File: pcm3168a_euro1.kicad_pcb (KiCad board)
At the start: 2 copper layers, 141.8 x 132.5 mm, 271 parts, among them J1 ACJS-MV35-3, J10 Conn_Coaxial, J11 Conn_Coaxial, J12 Conn_Coaxial, J13 Conn_Coaxial, J14 Conn_Coaxial, J15 Conn_Coaxial, J17 ACJS-MV35-3, J18 Conn_02x08_Odd_Even, J19 Conn_Coaxial, J21 ACJS-MV35-3, J22 ACJS-MV35-3, J24 ACJS-MV35-3, J25 ACJS-MV35-3, J26 ACJS-MV35-3, J27 ACJS-MV35-3, J8 Conn_01x02_Pin, J9 Conn_Coaxial, U1 PCM3168APAPR, U11 OPA1637, U12 TLV1117-33, U13 OPA1637, U14 OPA1637, U15 OPA1637, U16 OPA1637, U17 OPA1637, U18 OPA1637, U19 OPA1637, U2 74LVC1G17, U20 OPA1637, U21 OPA1637, U22 OPA1637, U23 OPA1637, U3 74LVC1G17, U4 74LVC1G17, U5 74LVC1G17, U6 74LVC1G17, U8 74LVC1G17, U9 74LVC1G17, Y1 SG-210STF 24.5760ML0

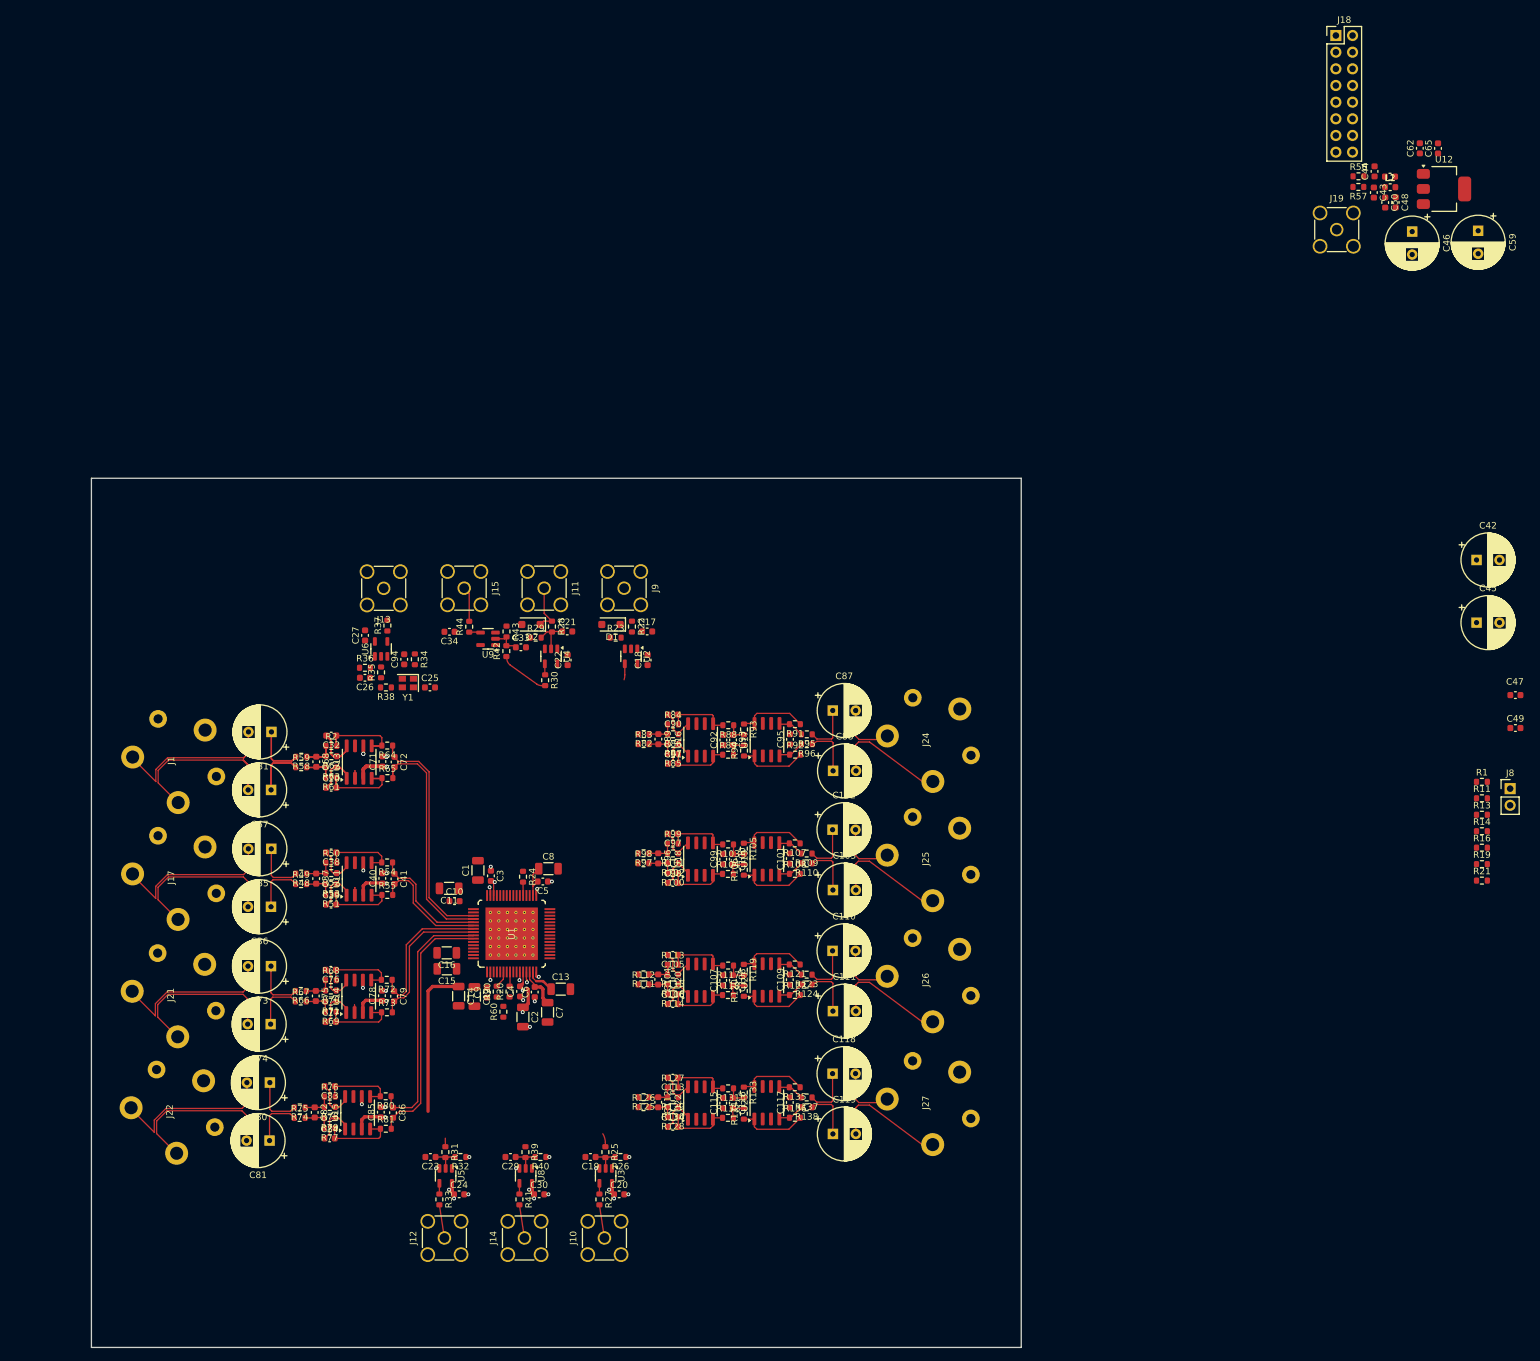
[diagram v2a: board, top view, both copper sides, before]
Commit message: WIP layout
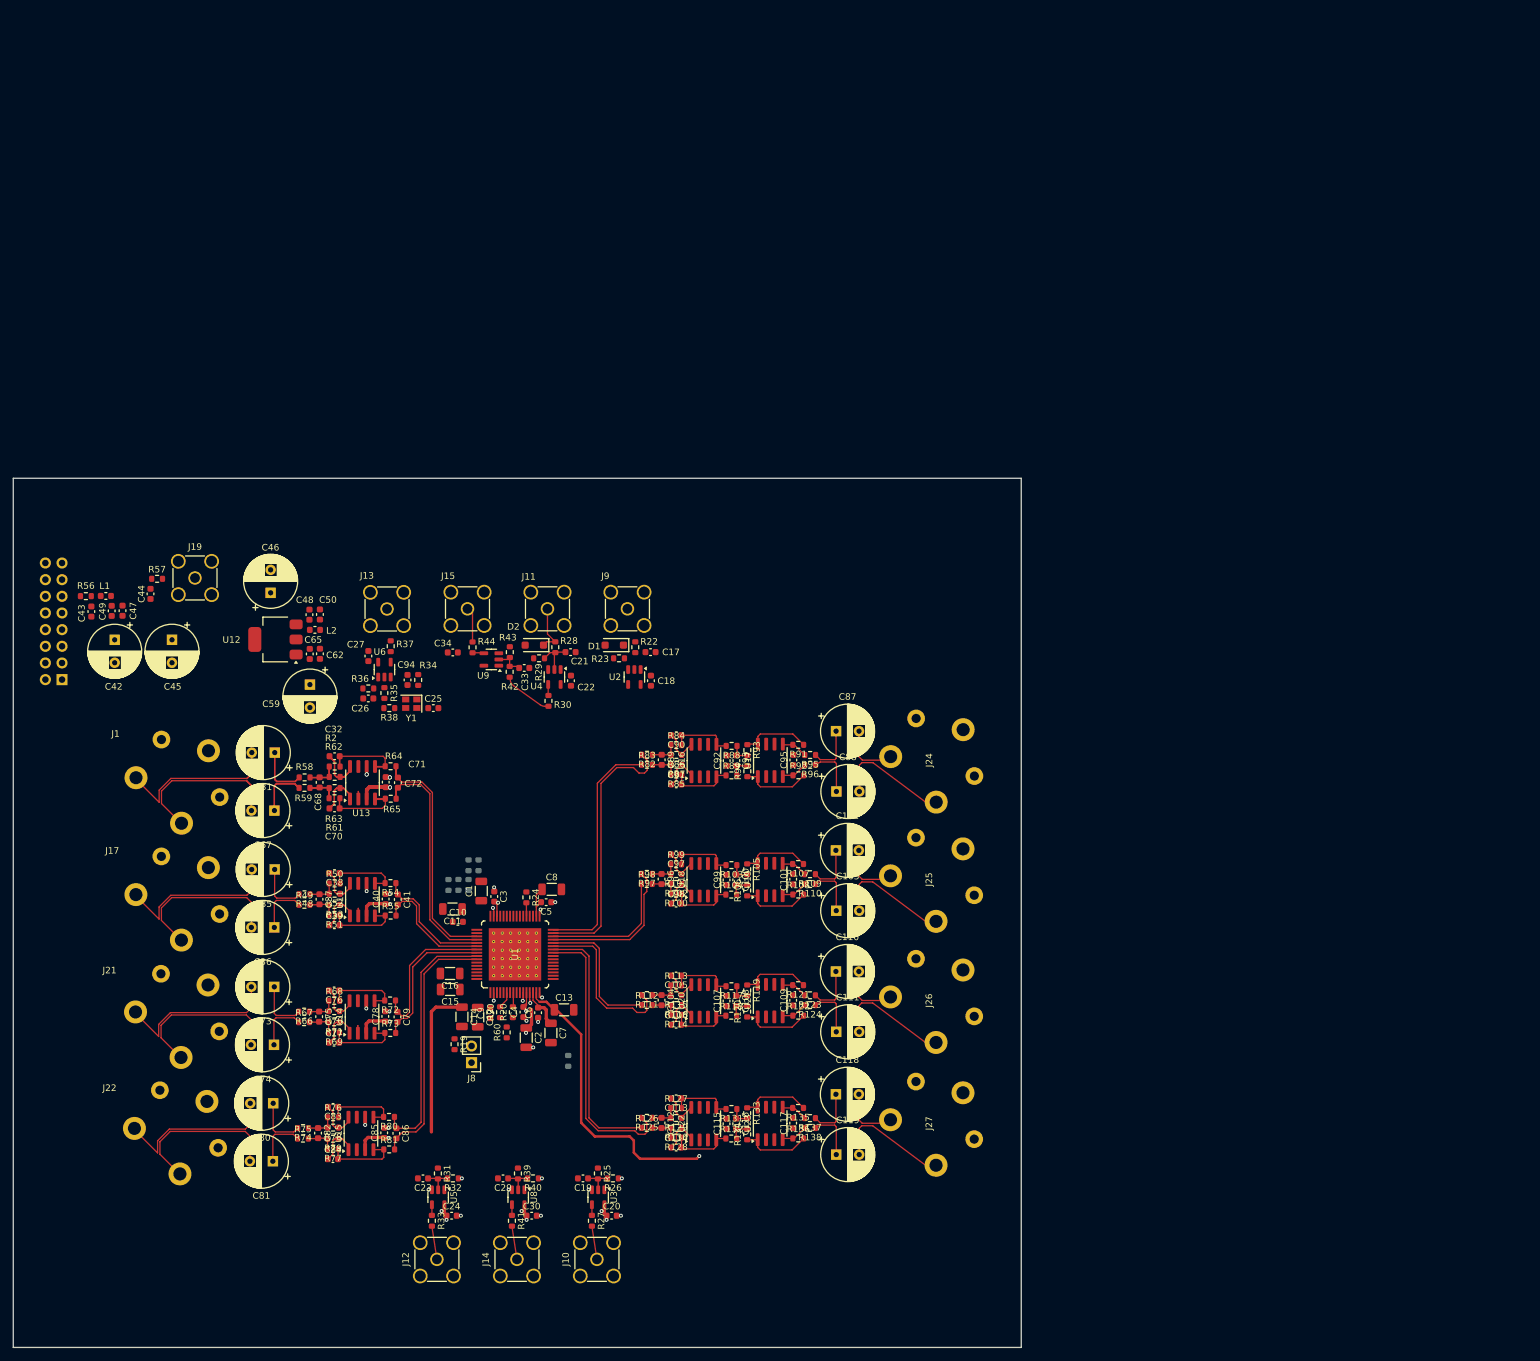
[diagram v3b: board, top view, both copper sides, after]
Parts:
- J18: footprint Connector_PinHeader_2.54mm:PinHeader_2x08_P2.54mm_Vertical -> Connector_PinSocket_2.54mm:PinSocket_2x08_P2.54mm_Vertical; moved to B.Cu
- R1, R11, R13, R14, R16, R21: moved to B.Cu
- moved J18 217.6 mm to (58.2, 115.2)
- moved C49 214.8 mm to (65.7, 104.7), turned to -90 degrees
- moved C47 212.7 mm to (67.4, 104.7), turned to -90 degrees
- moved C42 208.0 mm to (66.2, 109.1), turned to -90 degrees
- moved L1 206.0 mm to (64.8, 102.5)
- moved C43 205.7 mm to (62.6, 104.8)
- moved R56 204.3 mm to (61.8, 102.5)
- moved C45 198.9 mm to (74.9, 109.1), turned to -90 degrees
- moved C44 197.4 mm to (71.7, 102.1), turned to -90 degrees
- moved R57 192.6 mm to (72.7, 99.8), turned to 0 degrees
- moved C59 191.1 mm to (96.0, 116.0)
- moved U12 190.9 mm to (90.7, 109.1), turned to 180 degrees
- moved C65 188.5 mm to (95.9, 111.3), turned to -90 degrees
- moved C62 184.6 mm to (97.5, 111.3), turned to -90 degrees
- moved C46 182.5 mm to (90.0, 102.0), turned to 90 degrees
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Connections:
- C1 pad 1: +3.3V -> VDD
- C2 pad 1: +3.3V -> VDD
- C3 pad 2: +3.3V -> VDD
- C4 pad 2: +3.3V -> VDD
- C59 pad 1: +3.3V -> VDD
- C62 pad 1: +3.3V -> VDD
- C65 pad 1: +3.3V -> VDD
- U1 pad 12: +3.3V -> VDD
- U1 pad 46: +3.3V -> VDD
- U12 pad 2: +3.3V -> VDD
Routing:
- net /VOUT4+: track 0.00 -> 42.8 mm
- net /VOUT1+: track 0.00 -> 40.8 mm
- net Net-(U1-VCOMDA): track 4.39 -> 45.0 mm, vias 0 -> 1
- net /VOUT4-: track 0.00 -> 39.2 mm
- net /VOUT1-: track 0.00 -> 36.5 mm
- net /VOUT3+: track 0.00 -> 25.6 mm
- net /VOUT2+: track 0.00 -> 23.1 mm
- net /VOUT3-: track 0.00 -> 21.7 mm
- net /VOUT2-: track 0.00 -> 20.3 mm
- net +3.3V: track 9.95 -> 0.00 mm, vias 3 -> 0
- net VDD: track 8.64 -> 18.6 mm, vias 6 -> 9
- net Net-(R24-Pad1): track 2.45 -> 0.00 mm
- net /dout1/IN: track 2.04 -> 0.00 mm
- net /lrck_master/IN: track 1.30 -> 0.00 mm
- added copper zone on In2.Cu, net +5V
- added copper zone on In2.Cu, net VDD
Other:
- board size 141.8 x 132.5 mm -> 153.7 x 132.5 mm
- copper layers 2 -> 4

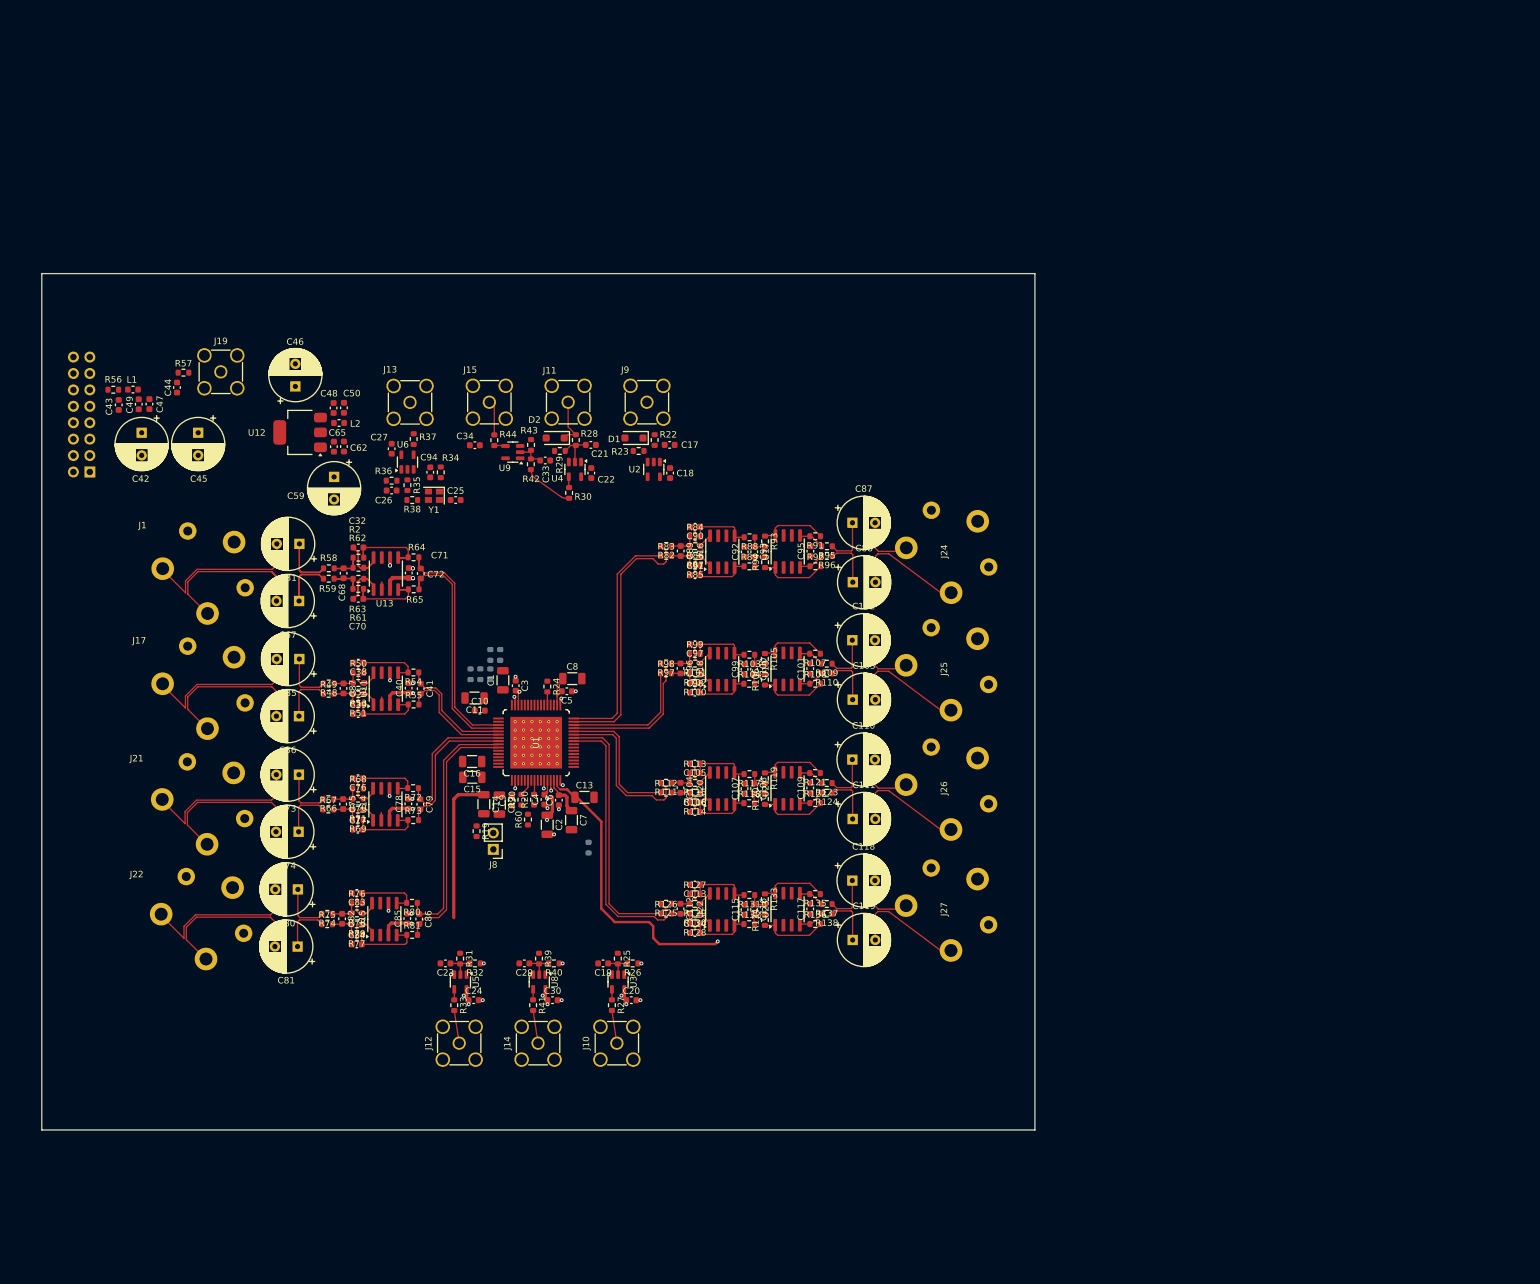
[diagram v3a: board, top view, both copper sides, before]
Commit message: WIP layout
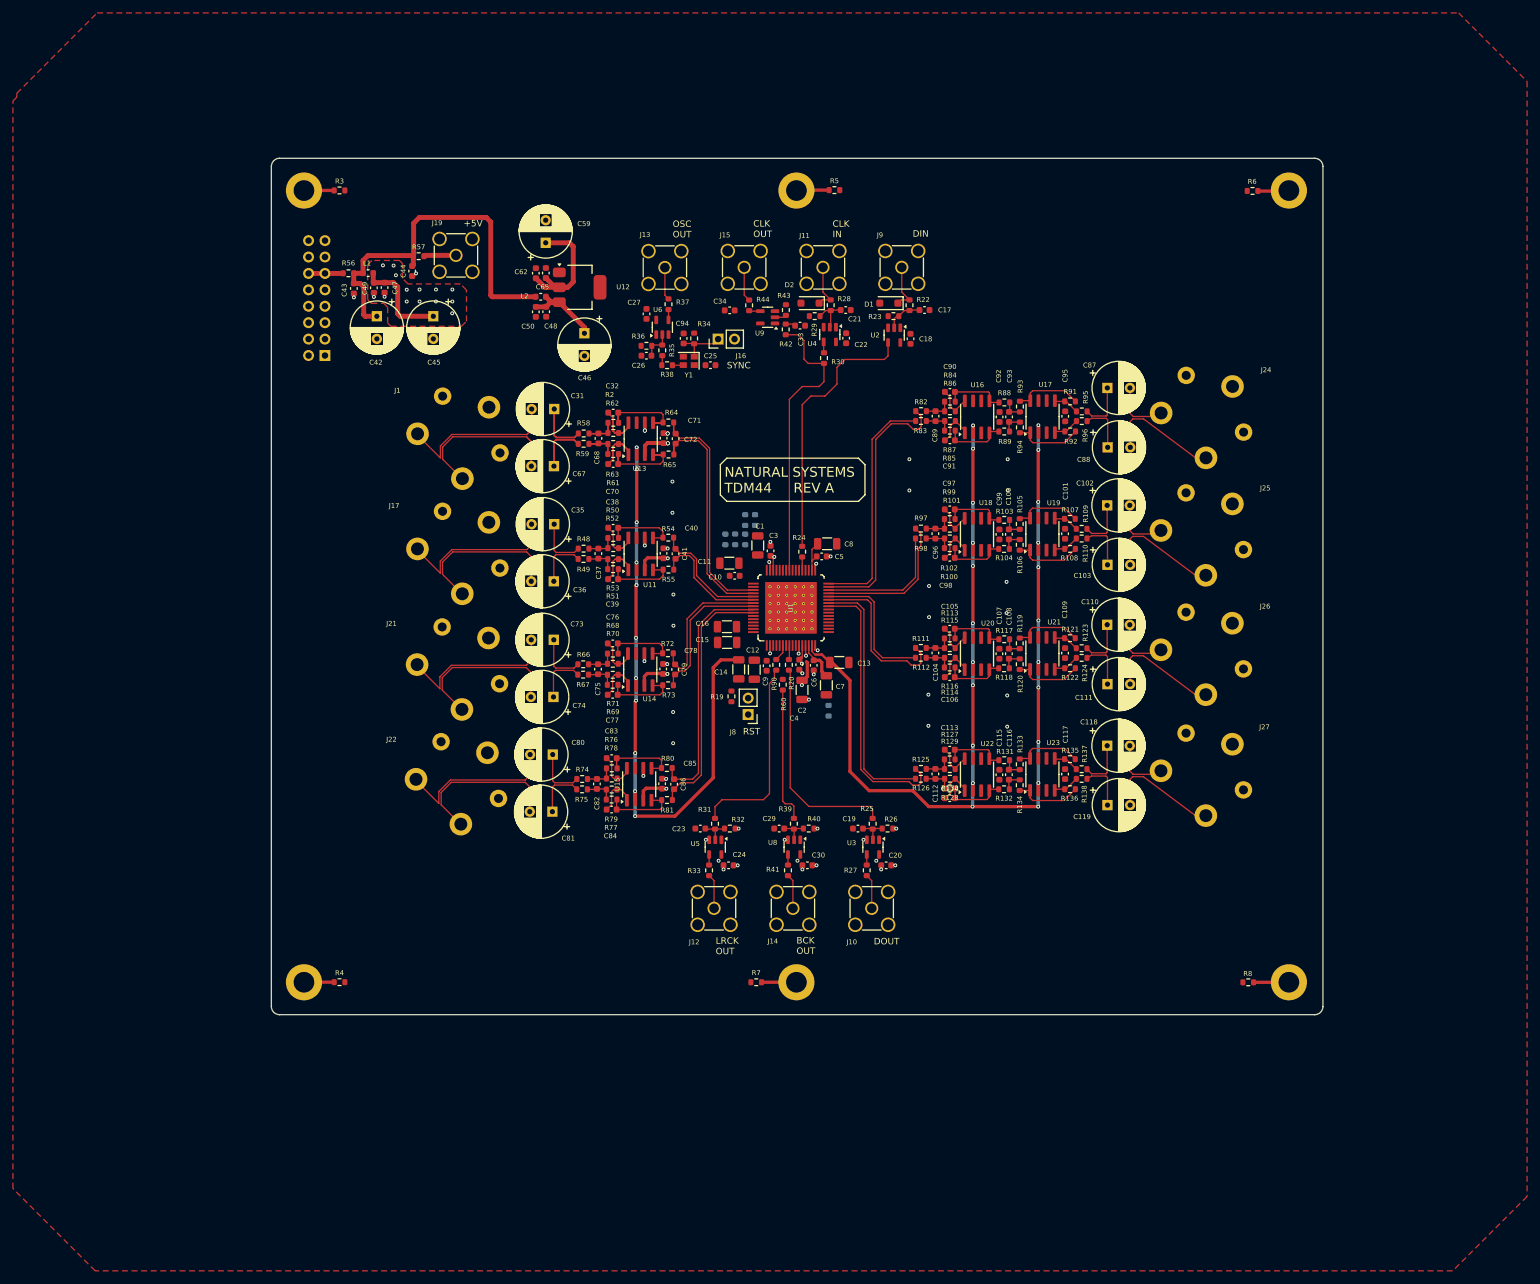
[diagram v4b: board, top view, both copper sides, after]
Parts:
- added H1: MountingHole_Pad, MountingHole:MountingHole_3.2mm_M3_DIN965_Pad, F.Cu at (91.3, 71.7)
- added H2: MountingHole_Pad, MountingHole:MountingHole_3.2mm_M3_DIN965_Pad, F.Cu at (91.3, 194.2)
- added H3: MountingHole_Pad, MountingHole:MountingHole_3.2mm_M3_DIN965_Pad, F.Cu at (167.5, 71.7)
- added H4: MountingHole_Pad, MountingHole:MountingHole_3.2mm_M3_DIN965_Pad, F.Cu at (243.7, 71.7)
- added H5: MountingHole_Pad, MountingHole:MountingHole_3.2mm_M3_DIN965_Pad, F.Cu at (167.5, 194.2)
- added H6: MountingHole_Pad, MountingHole:MountingHole_3.2mm_M3_DIN965_Pad, F.Cu at (243.7, 194.2)
- added J16: Conn_01x02_Pin, Connector_PinHeader_2.54mm:PinHeader_1x02_P2.54mm_Vertical, F.Cu at (155.4, 94.7)
- added R3: 0, Resistor_SMD:R_0603_1608Metric, F.Cu at (96.8, 71.7)
- added R4: 0, Resistor_SMD:R_0603_1608Metric, F.Cu at (96.8, 194.2)
- added R5: 0, Resistor_SMD:R_0603_1608Metric, F.Cu at (173.4, 71.6)
- added R6: 0, Resistor_SMD:R_0603_1608Metric, F.Cu at (238.1, 71.7)
- added R7: 0, Resistor_SMD:R_0603_1608Metric, F.Cu at (161.3, 194.2)
- added R8: 0, Resistor_SMD:R_0603_1608Metric, F.Cu at (237.4, 194.2)
- moved C59 48.8 mm to (128.7, 79.8), turned to 90 degrees
- moved U12 48.7 mm to (134.0, 86.6), turned to 0 degrees
- moved C46 45.5 mm to (134.7, 93.8), turned to -90 degrees
- moved C105 44.6 mm to (191.2, 139.5)
- moved C106 44.6 mm to (191.2, 147.0)
- moved C110 44.6 mm to (215.6, 138.8)
- moved C117 44.6 mm to (209.1, 162.0)
- moved C38 44.6 mm to (139.1, 123.9)
- moved C73 44.6 mm to (130.0, 141.2)
- moved C81 44.6 mm to (129.7, 167.8)
- moved C98 44.6 mm to (191.2, 128.5)
- moved J10 44.6 mm to (179.1, 182.7)
- moved J27 44.6 mm to (230.3, 162.0)
- moved J8 44.6 mm to (160.0, 152.7)
- moved R1 44.6 mm to (158.0, 125.6)
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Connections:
- C13 pad 1: Net-(U1-VCOMDA) -> VCOMDA
- U1 pad 15: Net-(U1-VCOMDA) -> VCOMDA
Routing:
- net VCOMDA: track 0.00 -> 172.2 mm, vias 0 -> 22
- net VCOMAD: track 26.8 -> 98.1 mm, vias 0 -> 11
- net Net-(C42-Pad1): track 0.00 -> 59.0 mm
- net Net-(U1-VCOMDA): track 45.0 -> 0.00 mm, vias 1 -> 0
- net Net-(R24-Pad1): track 0.00 -> 41.9 mm
- net /clk_in/OUT: track 7.83 -> 45.2 mm
- net /dout1/IN: track 0.00 -> 33.9 mm
- net /lrck_master/IN: track 0.00 -> 30.6 mm
- net /bck_master/IN: track 0.09 -> 21.2 mm
- net +5V: track 26.0 -> 41.4 mm, vias 5 -> 17
- net Net-(U12-VI): track 0.00 -> 12.8 mm
- net VDD: track 18.6 -> 29.3 mm
- net Net-(J16-Pin_1): track 0.00 -> 7.65 mm
- net Net-(D1-K): track 0.00 -> 7.53 mm
- net Net-(C17-Pad1): track 0.00 -> 5.87 mm
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- added copper zone on F.Cu, net +5V
- added copper zone on F.Cu, net GND
- added copper zone on In1.Cu, net GND
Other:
- board size 153.7 x 132.5 mm -> 162.7 x 132.5 mm
- board text added: "+5V"
- board text added: "BCK OUT"
- board text added: "CLK IN"
- board text added: "CLK OUT"
- board text added: "DIN"
- board text added: "DOUT"
- board text added: "LRCK OUT"
- board text added: "NATURAL SYSTEMS TDM44 REV A"
- board text added: "OSC OUT"
- board text added: "RST"
- board text added: "SYNC"
